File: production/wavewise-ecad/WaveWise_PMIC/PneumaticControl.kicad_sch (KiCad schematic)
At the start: 8 parts, among them K1 Relay_SPST-NO, Q2 2N2219, U1 Pololu_DRV8711_Motor_Driver

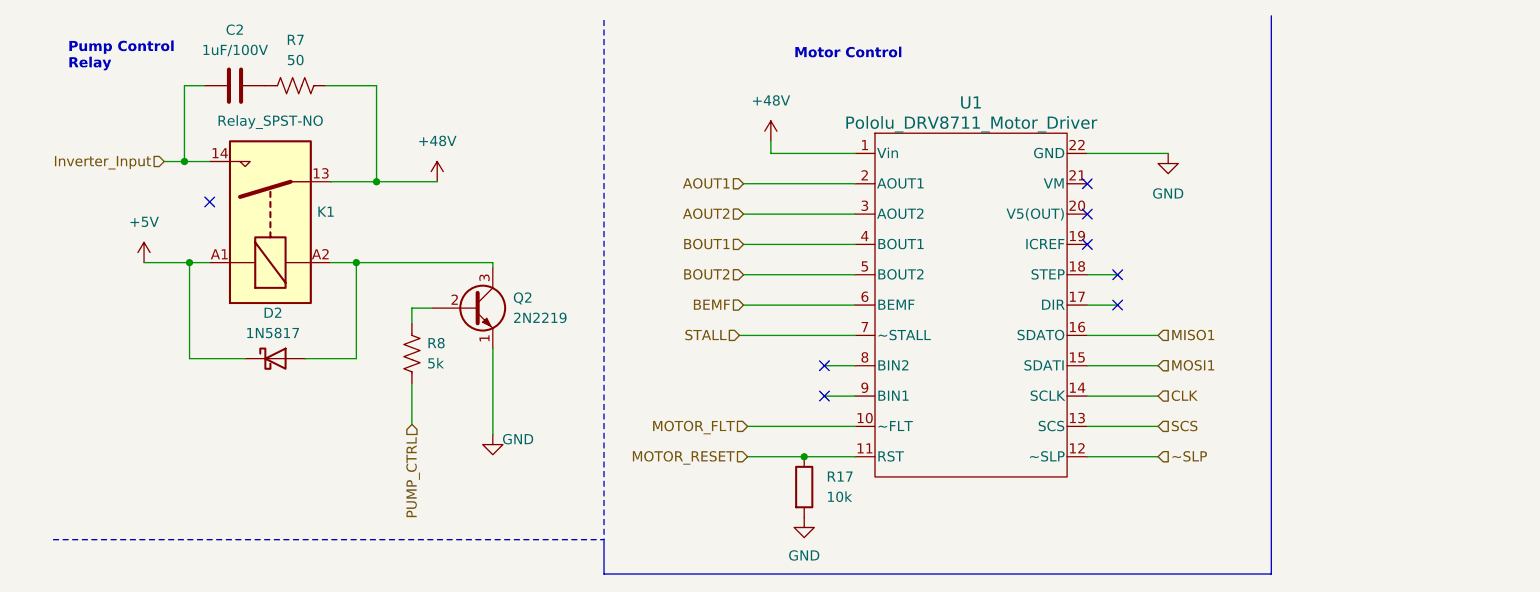
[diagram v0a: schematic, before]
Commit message: Prelim board layout
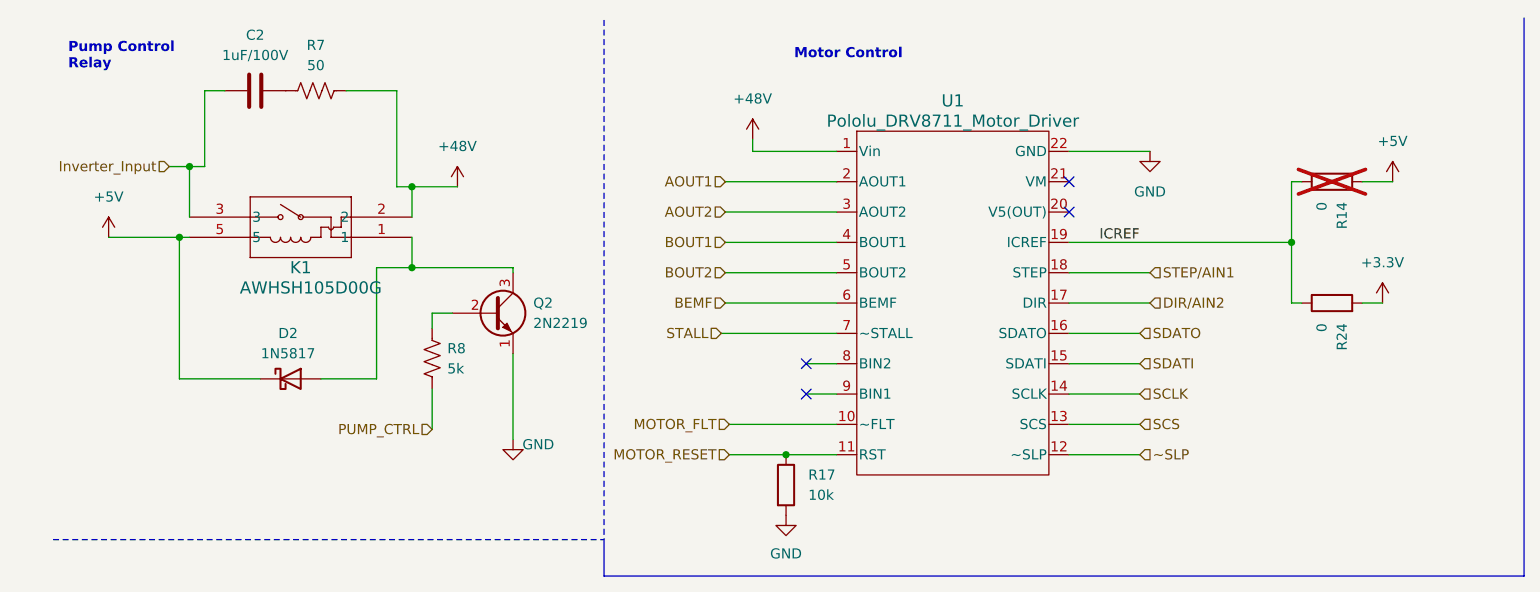
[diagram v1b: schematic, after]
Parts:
- removed K1: Relay_SPST-NO, Relay_THT:Relay_SPDT_Finder_36.11, symbol Relay:Relay_SPST-NO
- added K1: AWHSH105D00G, Unchecked:AWHSH105D00G, symbol AWHSH105D00G:AWHSH105D00G
- added R14, R24: 0, Resistor_SMD:R_0805_2012Metric, symbol Device:R
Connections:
- net +48V: now also K1.2
- net +5V: now also K1.5, R14.2
- net Inverter_Input: now also K1.3
- net at D2.2 (A), Q2.3 (C): now also K1.1
- net DIR/AIN2: now reaches U1.17 (DIR)
- net STEP/AIN1: now reaches U1.18 (STEP)
- net ICREF: now reaches U1.19 (ICREF)
- net ICREF: now also R14.1, R24.1
- net CLK renamed SCLK
- net MISO1 renamed SDATO
- net MOSI1 renamed SDATI
- new net +3.3V: R24.2
- no-connect marks 8 -> 4
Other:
- moved on the sheet: C2, D2, Q2, R17, R7, R8, U1

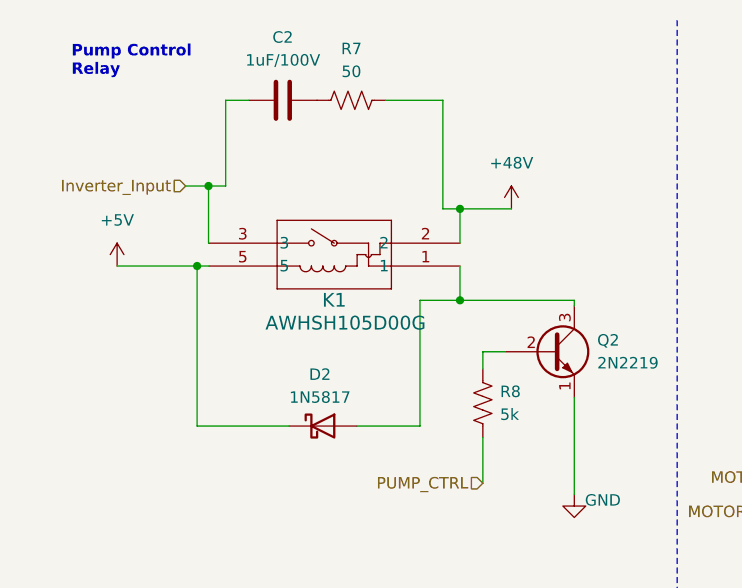
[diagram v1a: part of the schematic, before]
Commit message: power stuff
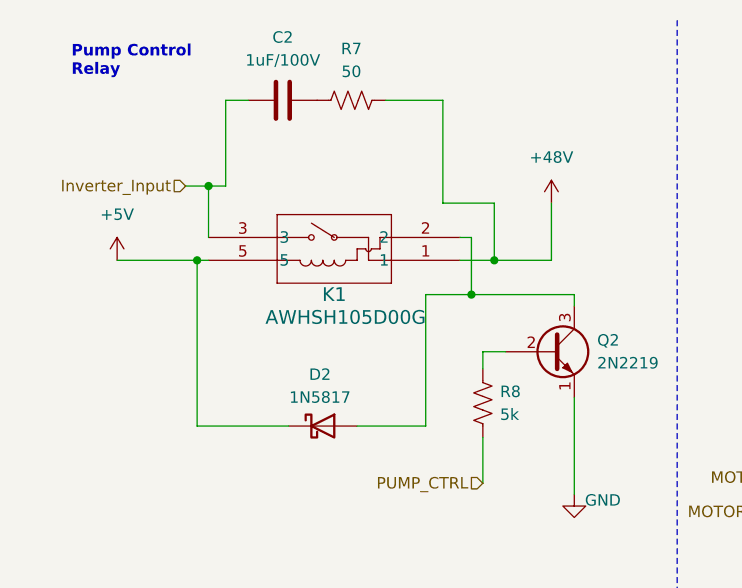
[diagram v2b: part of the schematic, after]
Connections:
- net +48V: now also K1.1; no longer K1.2
- net at D2.2 (A), Q2.3 (C): now also K1.2; no longer K1.1
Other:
- moved on the sheet: K1
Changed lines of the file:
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@@
   (junction (at 168.91 40.64) (diameter 0) (color 0 0 0 0)
   )
-  (junction (at 29.21 40.005) (diameter 0) (color 0 0 0 0)
-  )
-  (junction (at 58.42 43.815) (diameter 0) (color 0 0 0 0)
+  (junction (at 59.69 43.18) (diameter 0) (color 0 0 0 0)
   )
   (junction (at 105.41 67.31) (diameter 0) (color 0 0 0 0)
   )
-  (junction (at 58.42 33.655) (diameter 0) (color 0 0 0 0)
+  (junction (at 62.23 39.37) (diameter 0) (color 0 0 0 0)
+  )
+  (junction (at 29.21 39.37) (diameter 0) (color 0 0 0 0)
   )
   (junction (at 30.48 31.115) (diameter 0) (color 0 0 0 0)
@@
     (stroke (width 0) (type default))
   )
-  (wire (pts (xy 58.42 33.655) (xy 58.42 37.465))
-    (stroke (width 0) (type default))
-  )
   (wire (pts (xy 97.79 48.26) (xy 111.76 48.26))
     (stroke (width 0) (type default))
@@
     (stroke (width 0) (type default))
   )
+  (wire (pts (xy 68.58 39.37) (xy 62.23 39.37))
+    (stroke (width 0) (type default))
+  )
   (wire (pts (xy 140.97 63.5) (xy 149.86 63.5))
     (stroke (width 0) (type default))
   )
-  (wire (pts (xy 56.515 33.655) (xy 58.42 33.655))
+  (wire (pts (xy 56.515 33.02) (xy 62.23 33.02))
     (stroke (width 0) (type default))
   )
@@
     (stroke (width 0) (type default))
   )
-  (wire (pts (xy 53.975 43.815) (xy 58.42 43.815))
+  (wire (pts (xy 68.58 33.02) (xy 68.58 39.37))
     (stroke (width 0) (type default))
   )
@@
     (stroke (width 0) (type default))
   )
+  (wire (pts (xy 59.69 43.18) (xy 71.12 43.18))
+    (stroke (width 0) (type default))
+  )
   (wire (pts (xy 71.12 54.61) (xy 71.12 65.405))
     (stroke (width 0) (type default))
@@
     (stroke (width 0) (type default))
   )
+  (wire (pts (xy 59.69 36.83) (xy 59.69 43.18))
+    (stroke (width 0) (type default))
+  )
   (wire (pts (xy 140.97 52.07) (xy 149.86 52.07))
     (stroke (width 0) (type default))
   )
-  (wire (pts (xy 71.12 43.815) (xy 71.12 44.45))
-    (stroke (width 0) (type default))
-  )
   (wire (pts (xy 97.79 40.64) (xy 111.76 40.64))
     (stroke (width 0) (type default))
   )
-  (wire (pts (xy 29.21 40.005) (xy 29.21 57.785))
+  (wire (pts (xy 29.21 39.37) (xy 29.21 57.785))
     (stroke (width 0) (type default))
   )
@@
     (stroke (width 0) (type default))
   )
-  (wire (pts (xy 30.48 31.115) (xy 30.48 37.465))
+  (wire (pts (xy 30.48 31.115) (xy 30.48 36.83))
     (stroke (width 0) (type default))
   )
@@
     (stroke (width 0) (type default))
   )
-  (wire (pts (xy 58.42 43.815) (xy 71.12 43.815))
+  (wire (pts (xy 54.61 43.18) (xy 59.69 43.18))
     (stroke (width 0) (type default))
   )
@@
     (stroke (width 0) (type default))
   )
+  (wire (pts (xy 62.23 33.02) (xy 62.23 39.37))
+    (stroke (width 0) (type default))
+  )
   (wire (pts (xy 50.165 21.59) (xy 56.515 21.59))
     (stroke (width 0) (type default))
   )
-  (wire (pts (xy 58.42 33.655) (xy 64.135 33.655))
-    (stroke (width 0) (type default))
-  )
-  (wire (pts (xy 58.42 40.005) (xy 58.42 43.815))
-    (stroke (width 0) (type default))
-  )
   (wire (pts (xy 29.21 57.785) (xy 39.37 57.785))
     (stroke (width 0) (type default))
   )
-  (wire (pts (xy 46.99 57.785) (xy 53.975 57.785))
+  (wire (pts (xy 46.99 57.785) (xy 54.61 57.785))
     (stroke (width 0) (type default))
   )
@@
     (stroke (width 0.15) (type dash))
   )
+  (wire (pts (xy 62.23 39.37) (xy 58.42 39.37))
+    (stroke (width 0) (type default))
+  )
   (wire (pts (xy 32.385 21.59) (xy 32.385 31.115))
     (stroke (width 0) (type default))
@@
     (stroke (width 0) (type default))
   )
-  (wire (pts (xy 53.975 57.785) (xy 53.975 43.815))
-    (stroke (width 0) (type default))
-  )
-  (wire (pts (xy 56.515 21.59) (xy 56.515 33.655))
+  (wire (pts (xy 54.61 57.785) (xy 54.61 43.18))
+    (stroke (width 0) (type default))
+  )
+  (wire (pts (xy 56.515 21.59) (xy 56.515 33.02))
     (stroke (width 0) (type default))
   )
@@
     (stroke (width 0) (type default))
   )
-  (wire (pts (xy 20.32 40.005) (xy 29.21 40.005))
-    (stroke (width 0) (type default))
-  )
-  (wire (pts (xy 29.21 40.005) (xy 30.48 40.005))
+  (wire (pts (xy 20.32 39.37) (xy 29.21 39.37))
+    (stroke (width 0) (type default))
+  )
+  (wire (pts (xy 58.42 36.83) (xy 59.69 36.83))
+    (stroke (width 0) (type default))
+  )
+  (wire (pts (xy 71.12 43.18) (xy 71.12 44.45))
+    (stroke (width 0) (type default))
+  )
+  (wire (pts (xy 29.21 39.37) (xy 30.48 39.37))
     (stroke (width 0) (type default))
   )
@@
     )
   )
-  (symbol (lib_id "AWHSH105D00G:AWHSH105D00G") (at 58.42 40.005 180) (unit 1)
+  (symbol (lib_id "AWHSH105D00G:AWHSH105D00G") (at 58.42 39.37 180) (unit 1)
     (in_bom yes) (on_board yes) (dnp no)
-    (property "Reference" "K1" (at 44.45 43.815 0)
+    (property "Reference" "K1" (at 44.45 43.18 0)
       (effects (font (size 1.524 1.524)))
     )
-    (property "Value" "AWHSH105D00G" (at 45.72 46.355 0)
+    (property "Value" "AWHSH105D00G" (at 45.72 45.72 0)
       (effects (font (size 1.524 1.524)))
     )
-    (property "Footprint" "Unchecked:AWHSH105D00G" (at 58.42 40.005 0)
+    (property "Footprint" "Unchecked:AWHSH105D00G" (at 58.42 39.37 0)
       (effects (font (size 1.27 1.27) italic) hide)
     )
-    (property "Datasheet" "AWHSH105D00G" (at 58.42 40.005 0)
+    (property "Datasheet" "AWHSH105D00G" (at 58.42 39.37 0)
       (effects (font (size 1.27 1.27) italic) hide)
     )
@@
         (path "/ac491dca-bdaf-4a2e-a85e-04a34a1180ec"
           (reference "#PWR014") (unit 1)
-        )
-      )
-    )
-  )
-  (symbol (lib_id "power:+48V") (at 64.135 33.655 0) (unit 1)
-    (in_bom yes) (on_board yes) (dnp no) (fields_autoplaced)
-    (property "Reference" "#PWR02" (at 64.135 37.465 0)
-      (effects (font (size 1.27 1.27)) hide)
-    )
-    (property "Value" "+48V" (at 64.135 28.575 0)
-      (effects (font (size 1.27 1.27)))
-    )
-    (property "Footprint" "" (at 64.135 33.655 0)
-      (effects (font (size 1.27 1.27)) hide)
-    )
-    (property "Datasheet" "" (at 64.135 33.655 0)
-      (effects (font (size 1.27 1.27)) hide)
-    )
-    (pin "1")
-    (instances
-      (project "WaveWise_PMIC"
-        (path "/8343c01b-8940-4cb8-a17d-91fd7fb1cccd/9401b93a-998f-4185-ba4a-cb0793660d5a"
-          (reference "#PWR02") (unit 1)
         )
       )
@@
         (path "/8343c01b-8940-4cb8-a17d-91fd7fb1cccd/9401b93a-998f-4185-ba4a-cb0793660d5a"
           (reference "R8") (unit 1)
+        )
+      )
+    )
+  )
+  (symbol (lib_id "power:+48V") (at 68.58 33.02 0) (unit 1)
+    (in_bom yes) (on_board yes) (dnp no) (fields_autoplaced)
+    (property "Reference" "#PWR02" (at 68.58 36.83 0)
+      (effects (font (size 1.27 1.27)) hide)
+    )
+    (property "Value" "+48V" (at 68.58 27.94 0)
+      (effects (font (size 1.27 1.27)))
+    )
+    (property "Footprint" "" (at 68.58 33.02 0)
+      (effects (font (size 1.27 1.27)) hide)
+    )
+    (property "Datasheet" "" (at 68.58 33.02 0)
+      (effects (font (size 1.27 1.27)) hide)
+    )
+    (pin "1")
+    (instances
+      (project "WaveWise_PMIC"
+        (path "/8343c01b-8940-4cb8-a17d-91fd7fb1cccd/9401b93a-998f-4185-ba4a-cb0793660d5a"
+          (reference "#PWR02") (unit 1)
         )
       )
@@
     )
   )
-  (symbol (lib_id "power:+5V") (at 20.32 40.005 0) (unit 1)
-    (in_bom yes) (on_board yes) (dnp no) (fields_autoplaced)
-    (property "Reference" "#PWR07" (at 20.32 43.815 0)
-      (effects (font (size 1.27 1.27)) hide)
-    )
-    (property "Value" "+5V" (at 20.32 34.925 0)
-      (effects (font (size 1.27 1.27)))
-    )
-    (property "Footprint" "" (at 20.32 40.005 0)
-      (effects (font (size 1.27 1.27)) hide)
-    )
-    (property "Datasheet" "" (at 20.32 40.005 0)
-      (effects (font (size 1.27 1.27)) hide)
-    )
+  (symbol (lib_id "power:+5V") (at 20.32 39.37 0) (unit 1)
+    (in_bom yes) (on_board yes) (dnp no) (fields_autoplaced)
+    (property "Reference" "#PWR07" (at 20.32 43.18 0)
+      (effects (font (size 1.27 1.27)) hide)
+    )
+    (property "Value" "+5V" (at 20.32 34.29 0)
+      (effects (font (size 1.27 1.27)))
+    )
+    (property "Footprint" "" (at 20.32 39.37 0)
+      (effects (font (size 1.27 1.27)) hide)
+    )
+    (property "Datasheet" "" (at 20.32 39.37 0)
+      (effects (font (size 1.27 1.27)) hide)
+    )
